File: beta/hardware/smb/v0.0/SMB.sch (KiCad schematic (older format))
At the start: 21 parts, among them IC101 ATMEGA1284-A, J101 I2C, J102 RTS_RESET, J103 ICSP, J104 SERIAL_REV, SW101 reset_sw, X101 16MHz

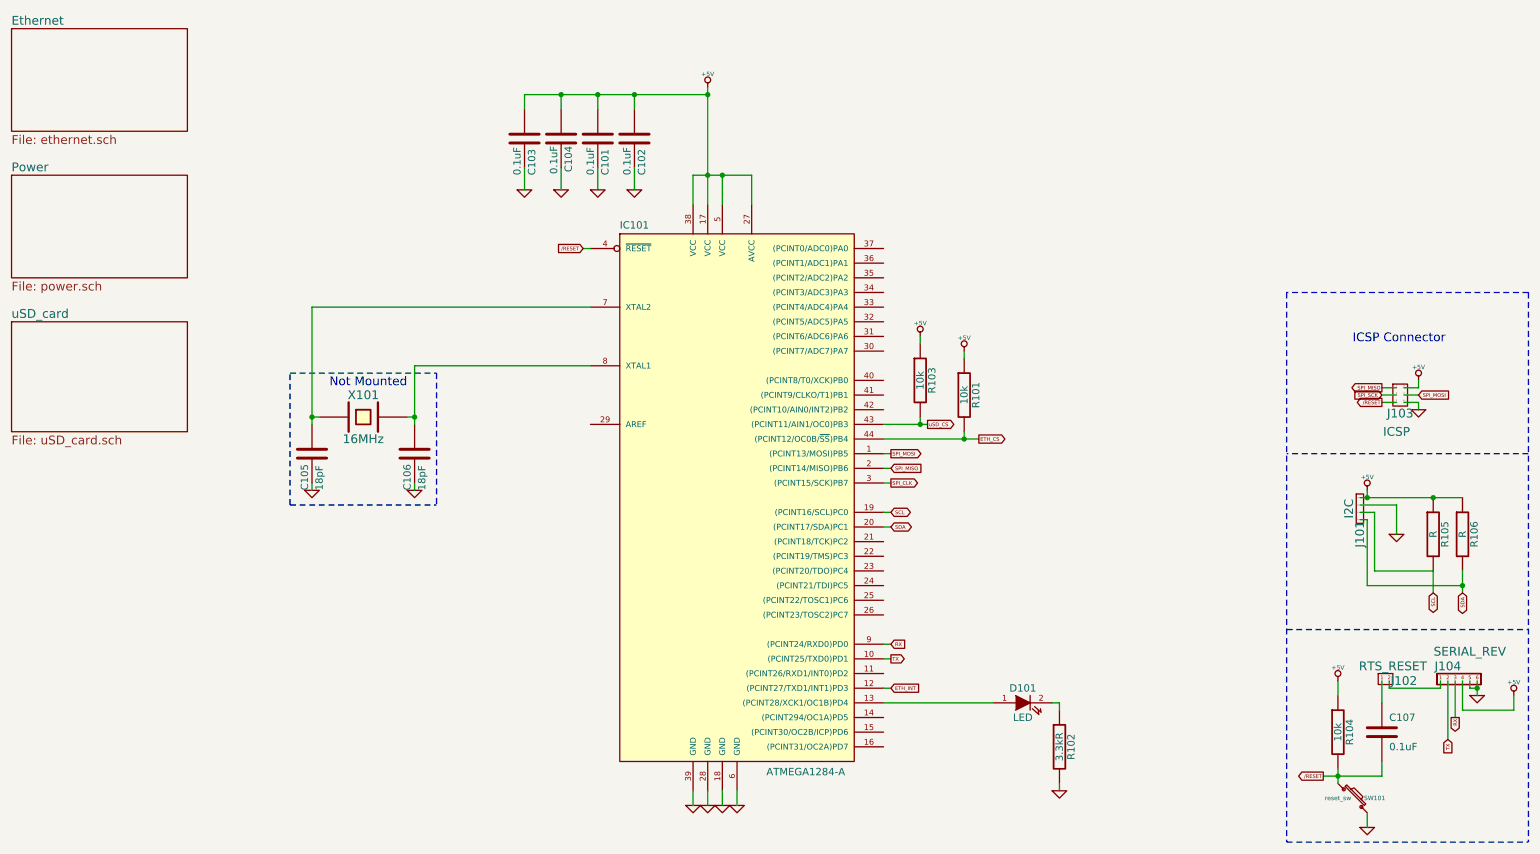
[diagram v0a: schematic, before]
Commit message: New components and corrections
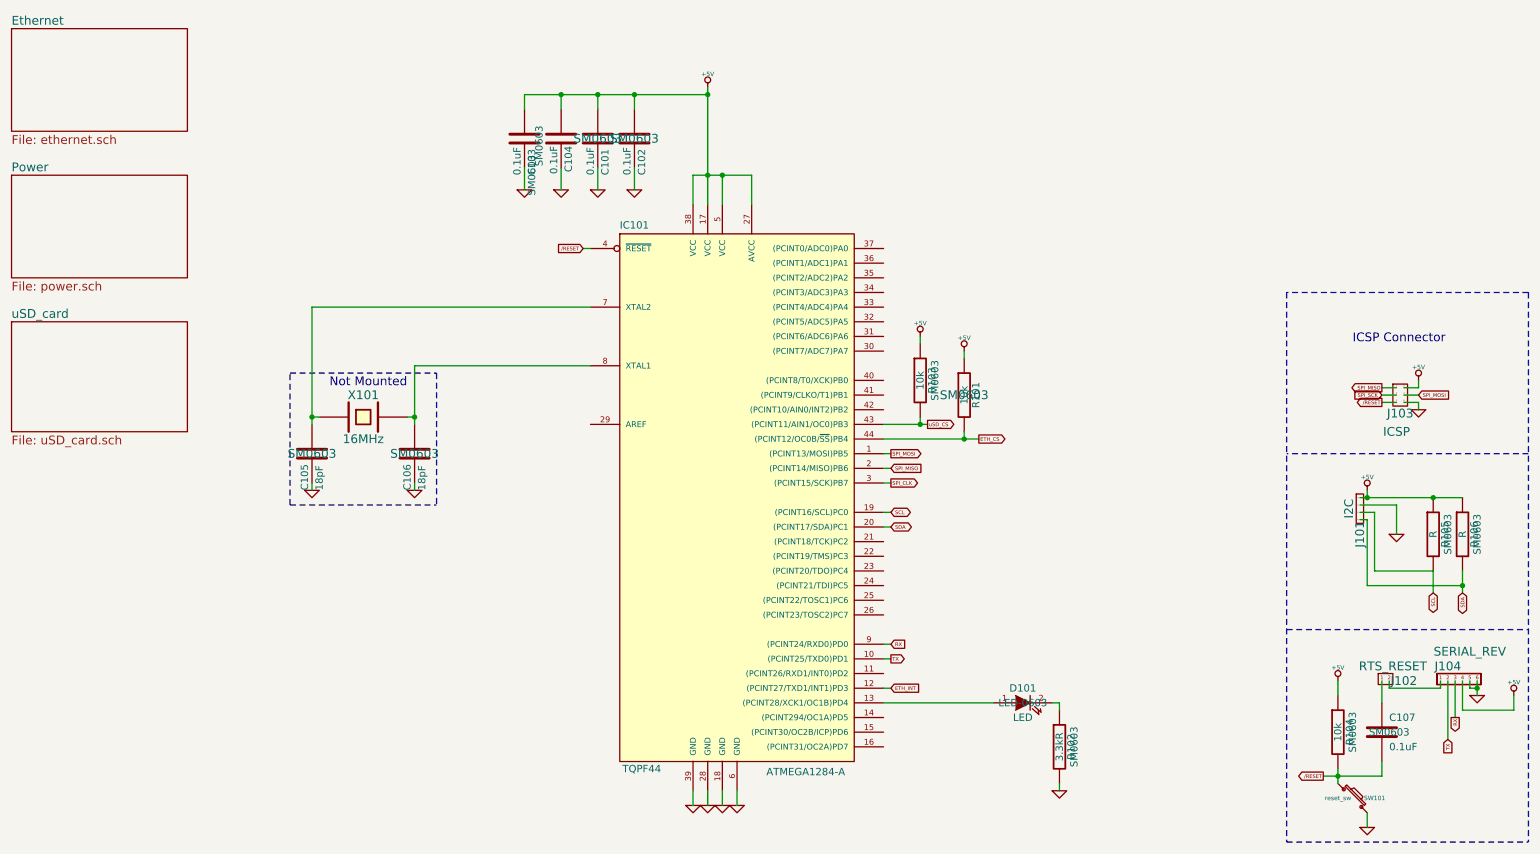
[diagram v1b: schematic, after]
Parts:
- C103, C104, C107, R102, R103, R104, R105, R106: footprint (none) -> SM0603
- D101: footprint (none) -> LED-0603
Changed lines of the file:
@@
-EESchema Schematic File Version 2  date 01/07/2012 23:30:37
+EESchema Schematic File Version 2  date 14/07/2012 20:45:27
 LIBS:power
 LIBS:device
@@
 LIBS:usd_conn
 LIBS:74lvc1g126gw
+LIBS:dual_self
 LIBS:SMB-cache
 EELAYER 25  0
@@
 Sheet 1 4
 Title ""
-Date "1 jul 2012"
+Date "14 jul 2012"
 Rev ""
 Comp ""
@@
 Connection ~ 6800 3300
 $Comp
-L +5V #PWR112
+L +5V #PWR01
 U 1 1 4FF09080
 P 6800 2700
-F 0 "#PWR112" H 6800 2790 20  0001 C CNN
+F 0 "#PWR01" H 6800 2790 20  0001 C CNN
 F 1 "+5V" H 6800 2790 30  0000 C CNN
 	1    6800 2700
@@
 F 0 "R103" V 6880 3000 50  0000 C CNN
 F 1 "10k" V 6800 3000 50  0000 C CNN
+F 2 "SM0603" V 6900 3000 50  0000 C CNN
 	1    6800 3000
 	1    0    0    -1
@@
 SPI_MOSI
 $Comp
-L +5V #PWR119
+L +5V #PWR02
 U 1 1 4FDE4559
 P 10200 3000
-F 0 "#PWR119" H 10200 3090 20  0001 C CNN
+F 0 "#PWR02" H 10200 3090 20  0001 C CNN
 F 1 "+5V" H 10200 3090 30  0000 C CNN
 	1    10200 3000
@@
 $EndComp
 $Comp
-L GND #PWR120
+L GND #PWR03
 U 1 1 4FDE454D
 P 10200 3200
-F 0 "#PWR120" H 10200 3200 30  0001 C CNN
+F 0 "#PWR03" H 10200 3200 30  0001 C CNN
 F 1 "GND" H 10200 3130 30  0001 C CNN
 	1    10200 3200
@@
 $EndSheet
 $Comp
-L +5V #PWR116
+L +5V #PWR04
 U 1 1 4FDE1B12
 P 9850 3750
-F 0 "#PWR116" H 9850 3840 20  0001 C CNN
+F 0 "#PWR04" H 9850 3840 20  0001 C CNN
 F 1 "+5V" H 9850 3840 30  0000 C CNN
 	1    9850 3750
@@
 $EndComp
 $Comp
-L +5V #PWR115
+L +5V #PWR05
 U 1 1 4FDE1B05
 P 9650 5050
-F 0 "#PWR115" H 9650 5140 20  0001 C CNN
+F 0 "#PWR05" H 9650 5140 20  0001 C CNN
 F 1 "+5V" H 9650 5140 30  0000 C CNN
 	1    9650 5050
@@
 $EndComp
 $Comp
-L +5V #PWR122
+L +5V #PWR06
 U 1 1 4FDE1B01
 P 10850 5150
-F 0 "#PWR122" H 10850 5240 20  0001 C CNN
+F 0 "#PWR06" H 10850 5240 20  0001 C CNN
 F 1 "+5V" H 10850 5240 30  0000 C CNN
 	1    10850 5150
@@
 $EndComp
 $Comp
-L +5V #PWR113
+L +5V #PWR07
 U 1 1 4FDE1AEF
 P 7100 2800
-F 0 "#PWR113" H 7100 2890 20  0001 C CNN
+F 0 "#PWR07" H 7100 2890 20  0001 C CNN
 F 1 "+5V" H 7100 2890 30  0000 C CNN
 	1    7100 2800
@@
 $EndComp
 $Comp
-L +5V #PWR108
+L +5V #PWR08
 U 1 1 4FDE1AE0
 P 5350 1000
-F 0 "#PWR108" H 5350 1090 20  0001 C CNN
+F 0 "#PWR08" H 5350 1090 20  0001 C CNN
 F 1 "+5V" H 5350 1090 30  0000 C CNN
 	1    5350 1000
@@
 $EndComp
 $Comp
-L GND #PWR109
+L GND #PWR09
 U 1 1 4FDE0BAB
 P 5350 5900
-F 0 "#PWR109" H 5350 5900 30  0001 C CNN
+F 0 "#PWR09" H 5350 5900 30  0001 C CNN
 F 1 "GND" H 5350 5830 30  0001 C CNN
 	1    5350 5900
@@
 $EndComp
 $Comp
-L GND #PWR107
+L GND #PWR010
 U 1 1 4FDE0BA8
 P 5250 5900
-F 0 "#PWR107" H 5250 5900 30  0001 C CNN
+F 0 "#PWR010" H 5250 5900 30  0001 C CNN
 F 1 "GND" H 5250 5830 30  0001 C CNN
 	1    5250 5900
@@
 $EndComp
 $Comp
-L GND #PWR110
+L GND #PWR011
 U 1 1 4FDE0BA5
 P 5450 5900
-F 0 "#PWR110" H 5450 5900 30  0001 C CNN
+F 0 "#PWR011" H 5450 5900 30  0001 C CNN
 F 1 "GND" H 5450 5830 30  0001 C CNN
 	1    5450 5900
@@
 $EndComp
 $Comp
-L GND #PWR111
+L GND #PWR012
 U 1 1 4FDE0BA2
 P 5550 5900
-F 0 "#PWR111" H 5550 5900 30  0001 C CNN
+F 0 "#PWR012" H 5550 5900 30  0001 C CNN
 F 1 "GND" H 5550 5830 30  0001 C CNN
 	1    5550 5900
@@
 $EndComp
 $Comp
-L GND #PWR106
+L GND #PWR013
 U 1 1 4FDE09A7
 P 4850 1700
-F 0 "#PWR106" H 4850 1700 30  0001 C CNN
+F 0 "#PWR013" H 4850 1700 30  0001 C CNN
 F 1 "GND" H 4850 1630 30  0001 C CNN
 	1    4850 1700
@@
 $EndComp
 $Comp
-L GND #PWR105
+L GND #PWR014
 U 1 1 4FDE09A4
 P 4600 1700
-F 0 "#PWR105" H 4600 1700 30  0001 C CNN
+F 0 "#PWR014" H 4600 1700 30  0001 C CNN
 F 1 "GND" H 4600 1630 30  0001 C CNN
 	1    4600 1700
@@
 $EndComp
 $Comp
-L GND #PWR104
+L GND #PWR015
 U 1 1 4FDE09A1
 P 4350 1700
-F 0 "#PWR104" H 4350 1700 30  0001 C CNN
+F 0 "#PWR015" H 4350 1700 30  0001 C CNN
 F 1 "GND" H 4350 1630 30  0001 C CNN
 	1    4350 1700
@@
 $EndComp
 $Comp
-L GND #PWR103
+L GND #PWR016
 U 1 1 4FDE099C
 P 4100 1700
-F 0 "#PWR103" H 4100 1700 30  0001 C CNN
+F 0 "#PWR016" H 4100 1700 30  0001 C CNN
 F 1 "GND" H 4100 1630 30  0001 C CNN
 	1    4100 1700
@@
 F 0 "C103" V 4150 1100 50  0000 L CNN
 F 1 "0.1uF" V 4050 1100 50  0000 L CNN
+F 2 "SM0603" V 4150 1100 50  0000 C CNN
 	1    4100 1350
 	1    0    0    -1
@@
 F 0 "IC101" H 4750 5630 50  0000 L BNN
 F 1 "ATMEGA1284-A" H 5750 1900 50  0000 L BNN
-F 2 "TQPF44" H 4900 1950 50  0001 C CNN
+F 2 "TQPF44" H 4900 1950 50  0000 C CNN
 	1    5550 3800
 	1    0    0    -1
@@
 SDA
 $Comp
-L GND #PWR118
+L GND #PWR017
 U 1 1 4FA06DB4
 P 10050 4050
-F 0 "#PWR118" H 10050 4050 30  0001 C CNN
+F 0 "#PWR017" H 10050 4050 30  0001 C CNN
 F 1 "GND" H 10050 3980 30  0001 C CNN
 	1    10050 4050
@@
 F 0 "R106" V 10580 4050 50  0000 C CNN
 F 1 "R" V 10500 4050 50  0000 C CNN
+F 2 "SM0603" V 10600 4050 50  0000 C CNN
 	1    10500 4050
 	1    0    0    -1
@@
 F 0 "R105" V 10380 4050 50  0000 C CNN
 F 1 "R" V 10300 4050 50  0000 C CNN
+F 2 "SM0603" V 10400 4050 50  0000 C CNN
 	1    10300 4050
 	1    0    0    -1
@@
 F 0 "R101" V 7180 3100 50  0000 C CNN
 F 1 "10k" V 7100 3100 50  0000 C CNN
-F 2 "SM0603" H 7100 3100 60  0001 C CNN
+F 2 "SM0603" H 7100 3100 60  0000 C CNN
 	1    7100 3100
 	1    0    0    -1
@@
 TX
 $Comp
-L GND #PWR121
+L GND #PWR018
 U 1 1 4FA025EE
 P 10600 5150
-F 0 "#PWR121" H 10600 5150 30  0001 C CNN
+F 0 "#PWR018" H 10600 5150 30  0001 C CNN
 F 1 "GND" H 10600 5080 30  0001 C CNN
 	1    10600 5150
@@
 F 0 "C107" H 10000 5500 50  0000 L CNN
 F 1 "0.1uF" H 10000 5300 50  0000 L CNN
+F 2 "SM0603" H 10000 5400 50  0000 C CNN
 	1    9950 5400
 	1    0    0    -1
@@
 /RESET
 $Comp
-L GND #PWR117
+L GND #PWR019
 U 1 1 4FA01B14
 P 9850 6050
-F 0 "#PWR117" H 9850 6050 30  0001 C CNN
+F 0 "#PWR019" H 9850 6050 30  0001 C CNN
 F 1 "GND" H 9850 5980 30  0001 C CNN
 	1    9850 6050
@@
 F 0 "R104" V 9730 5400 50  0000 C CNN
 F 1 "10k" V 9650 5400 50  0000 C CNN
+F 2 "SM0603" V 9750 5400 50  0000 C CNN
 	1    9650 5400
 	1    0    0    -1
@@
 /RESET
 $Comp
-L GND #PWR114
+L GND #PWR020
 U 1 1 4FA01A42
 P 7750 5800
-F 0 "#PWR114" H 7750 5800 30  0001 C CNN
+F 0 "#PWR020" H 7750 5800 30  0001 C CNN
 F 1 "GND" H 7750 5730 30  0001 C CNN
 	1    7750 5800
@@
 F 0 "R102" V 7830 5500 50  0000 C CNN
 F 1 "3.3kR" V 7750 5500 50  0000 C CNN
+F 2 "SM0603" V 7850 5500 50  0000 C CNN
 	1    7750 5500
 	1    0    0    -1
@@
 F 0 "D101" H 7500 5300 50  0000 C CNN
 F 1 "LED" H 7500 5100 50  0000 C CNN
+F 2 "LED-0603" H 7500 5200 50  0000 C CNN
 	1    7500 5200
 	1    0    0    -1
@@
 F 0 "C104" V 4300 1400 50  0000 L CNN
 F 1 "0.1uF" V 4400 1400 50  0000 L CNN
+F 2 "SM0603" V 4500 1400 50  0000 C CNN
 	1    4350 1350
 	-1   0    0    1
 $EndComp
 $Comp
-L GND #PWR102
+L GND #PWR021
 U 1 1 4FA01409
 P 3350 3750
-F 0 "#PWR102" H 3350 3750 30  0001 C CNN
+F 0 "#PWR021" H 3350 3750 30  0001 C CNN
 F 1 "GND" H 3350 3680 30  0001 C CNN
 	1    3350 3750
@@
 $EndComp
 $Comp
-L GND #PWR101
+L GND #PWR022
 U 1 1 4FA01406
 P 2650 3750
-F 0 "#PWR101" H 2650 3750 30  0001 C CNN
+F 0 "#PWR022" H 2650 3750 30  0001 C CNN
 F 1 "GND" H 2650 3680 30  0001 C CNN
 	1    2650 3750
@@
 F 0 "C106" V 3300 3250 50  0000 L CNN
 F 1 "18pF" V 3400 3250 50  0000 L CNN
-F 2 "SM0603" H 3350 3500 60  0001 C CNN
+F 2 "SM0603" H 3350 3500 60  0000 C CNN
 	1    3350 3500
 	1    0    0    -1
@@
 F 0 "C105" V 2600 3250 50  0000 L CNN
 F 1 "18pF" V 2700 3250 50  0000 L CNN
-F 2 "SM0603" H 2650 3500 60  0001 C CNN
+F 2 "SM0603" H 2650 3500 60  0000 C CNN
 	1    2650 3500
 	1    0    0    -1
@@
 F 0 "C102" V 4900 1100 50  0000 L CNN
 F 1 "0.1uF" V 4800 1100 50  0000 L CNN
-F 2 "SM0603" H 4850 1350 60  0001 C CNN
+F 2 "SM0603" H 4850 1350 60  0000 C CNN
 	1    4850 1350
 	1    0    0    -1
@@
 F 0 "C101" V 4650 1100 50  0000 L CNN
 F 1 "0.1uF" V 4550 1100 50  0000 L CNN
-F 2 "SM0603" H 4600 1350 60  0001 C CNN
+F 2 "SM0603" H 4600 1350 60  0000 C CNN
 	1    4600 1350
 	1    0    0    -1
